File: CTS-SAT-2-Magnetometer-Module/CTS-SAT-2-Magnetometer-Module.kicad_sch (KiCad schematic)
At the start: 31 parts, among them J2 SWD, J3 I2C, SW1 SW_Push, U1 MMC5983MA, U2 LIS2MDL, U3 STM32F072C8Tx, U5 MIC5365-3.0YC5

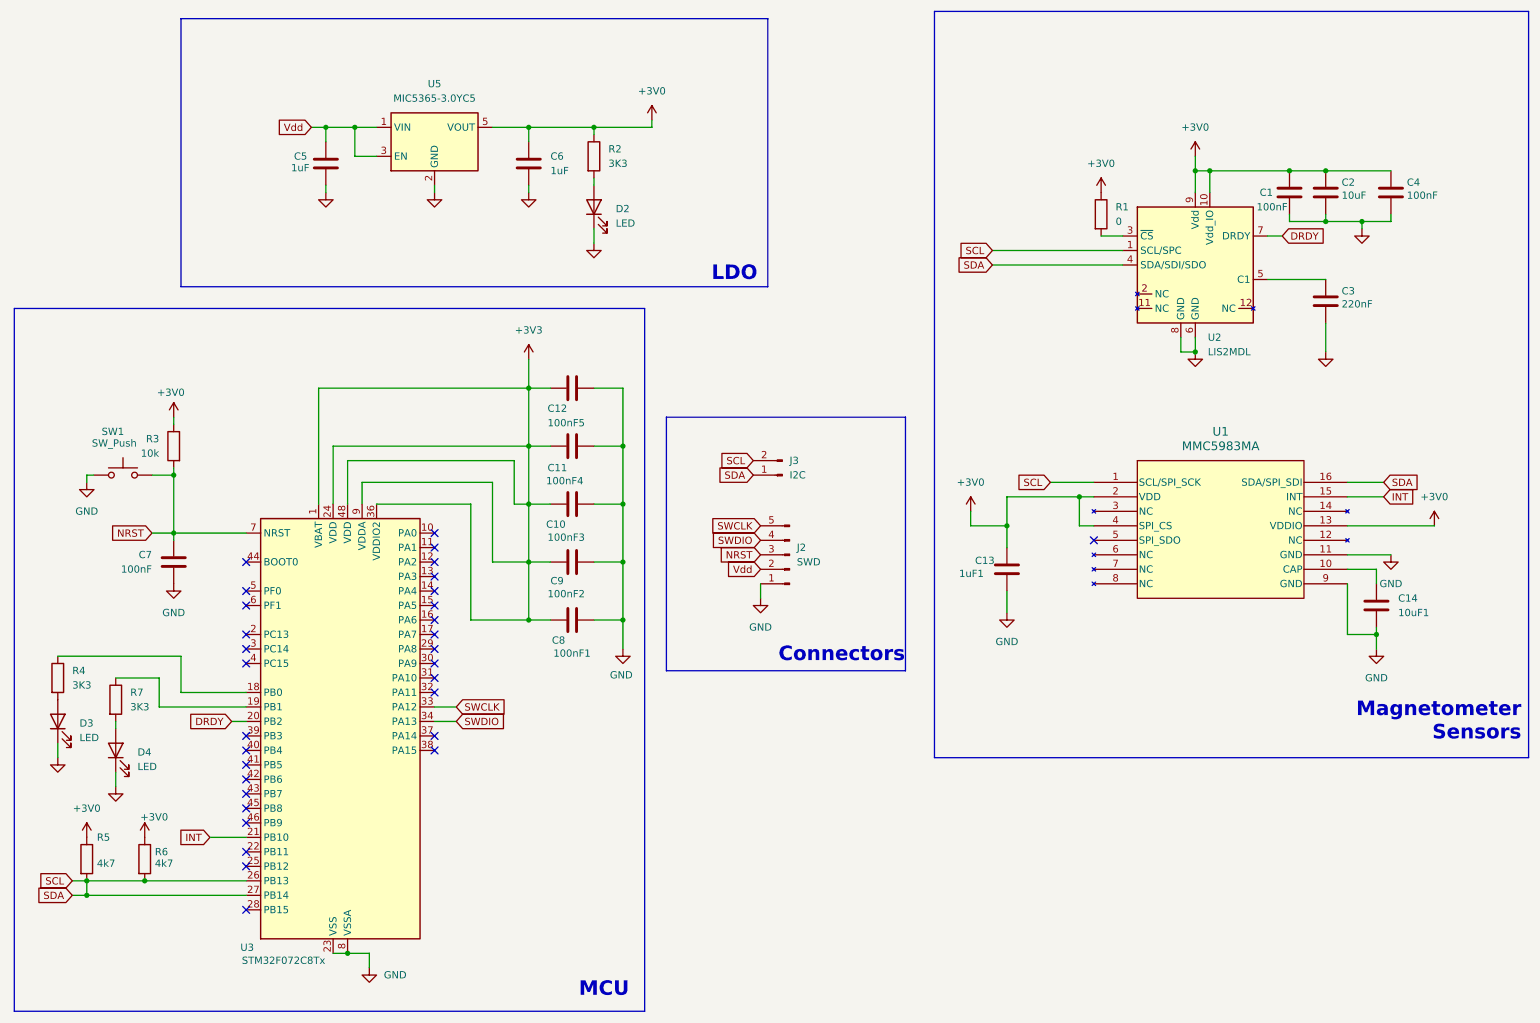
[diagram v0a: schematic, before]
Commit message: Applied Changes following Review 2
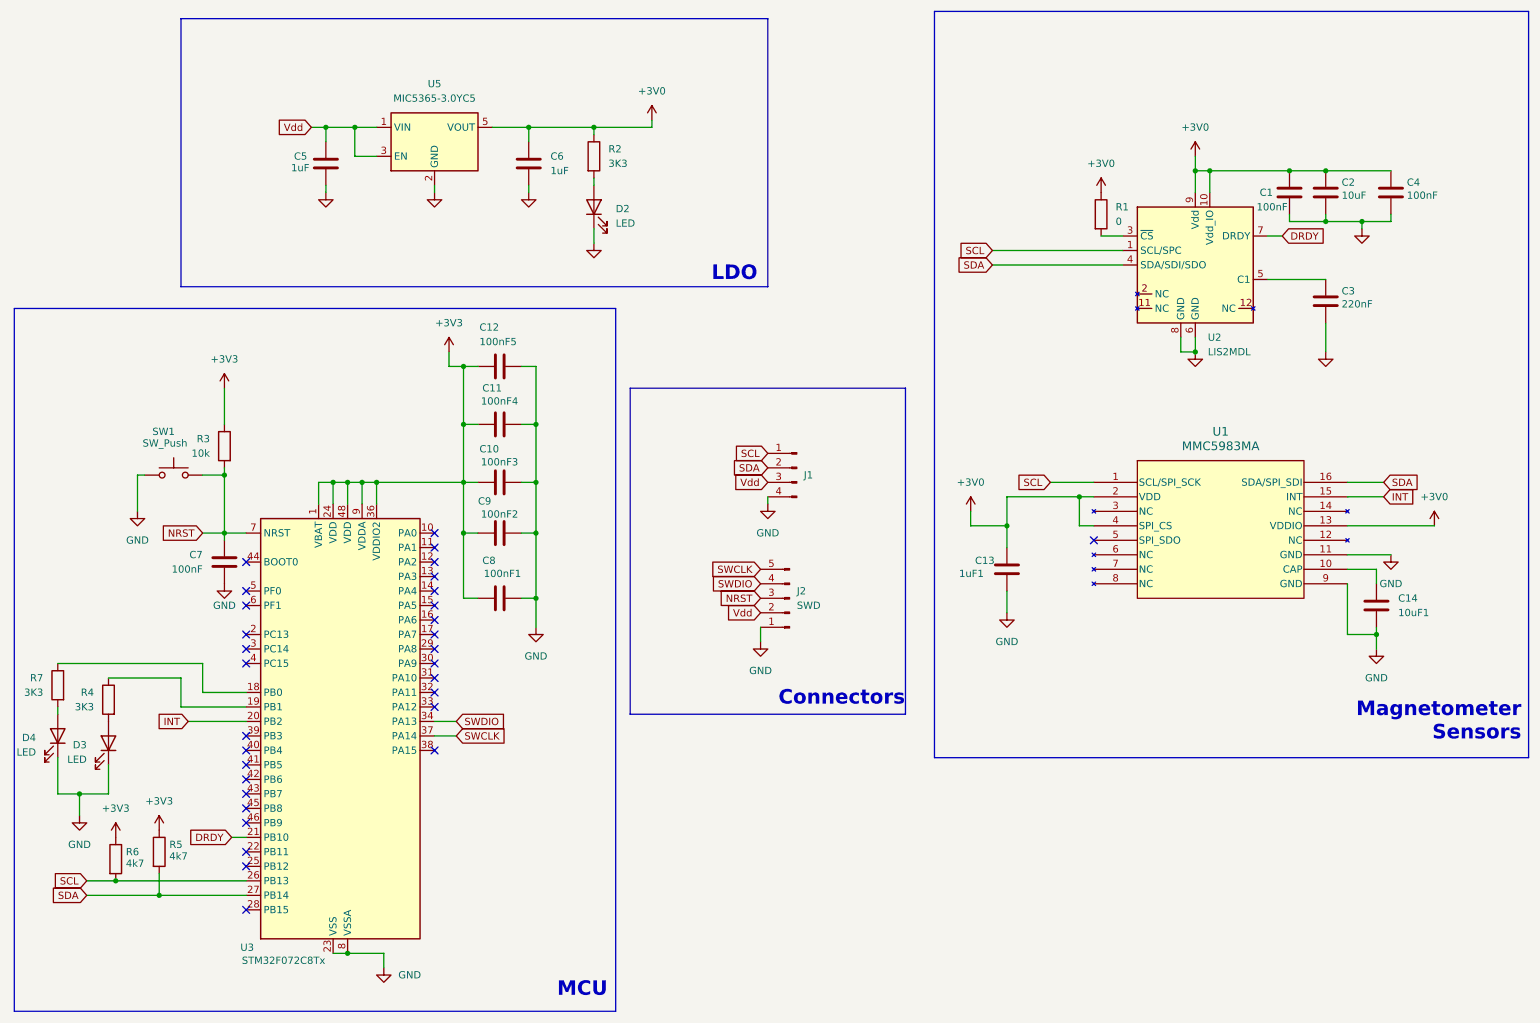
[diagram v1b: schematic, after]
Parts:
- removed J3: I2C, Connector_PinHeader_2.54mm:PinHeader_1x02_P2.54mm_Vertical, symbol Connector:Conn_01x02_Pin
- added J1: Conn_01x04_Pin, symbol Connector:Conn_01x04_Pin
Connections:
- net +3V0: no longer R3.1, R5.1, R6.1
- net +3V3: now also C10.1, C9.2, R3.1, R5.1, R6.1; no longer C10.2, C9.1
- net DRDY: now also U3.21 (PB10); no longer U3.20 (PB2)
- net GND: now also C10.2, C9.1, J1.4 (Pin_4); no longer C10.1, C9.2
- net INT: now also U3.20 (PB2); no longer U3.21 (PB10)
- net SCL: now also J1.1 (Pin_1); no longer R5.2, U1.16 (SDA/SPI_SDI), U2.4 (SDA/SDI/SDO), U3.27 (PB14)
- net SWCLK: now also U3.37 (PA14); no longer U3.33 (PA12)
- net Vdd: now also J1.3 (Pin_3)
- net at U3.18 (PB0): now also R7.1; no longer R4.1
- net at U3.19 (PB1): now also R4.1; no longer R7.1
- new net SDA: J1.2 (Pin_2), R5.2, U1.16 (SDA/SPI_SDI), U2.4 (SDA/SDI/SDO), U3.27 (PB14)
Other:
- moved on the sheet: C10, C11, C12, C7, C8, C9, D3, D4, J2, R3, R4, R5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

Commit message: started pcb
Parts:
- J1: footprint (none) -> Connector_PinHeader_2.54mm:PinHeader_1x04_P2.54mm_Vertical
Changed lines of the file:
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@@
 			)
 		)
-		(property "Footprint" ""
+		(property "Footprint" "Connector_PinHeader_2.54mm:PinHeader_1x04_P2.54mm_Vertical"
 			(at 154.94 97.79 0)
 			(hide yes)
